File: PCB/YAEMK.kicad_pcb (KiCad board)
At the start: 2 copper layers, 162.8 x 130.8 mm, 177 parts, among them J1 DBG, P1 PC, P2 Link, P3 SSD1107, Q1 SSP6206, SW1 ALPS EC11, U1 USBLC6-2SC6, U2 USBLC6-2SC6, U3 STM32F103CBTx

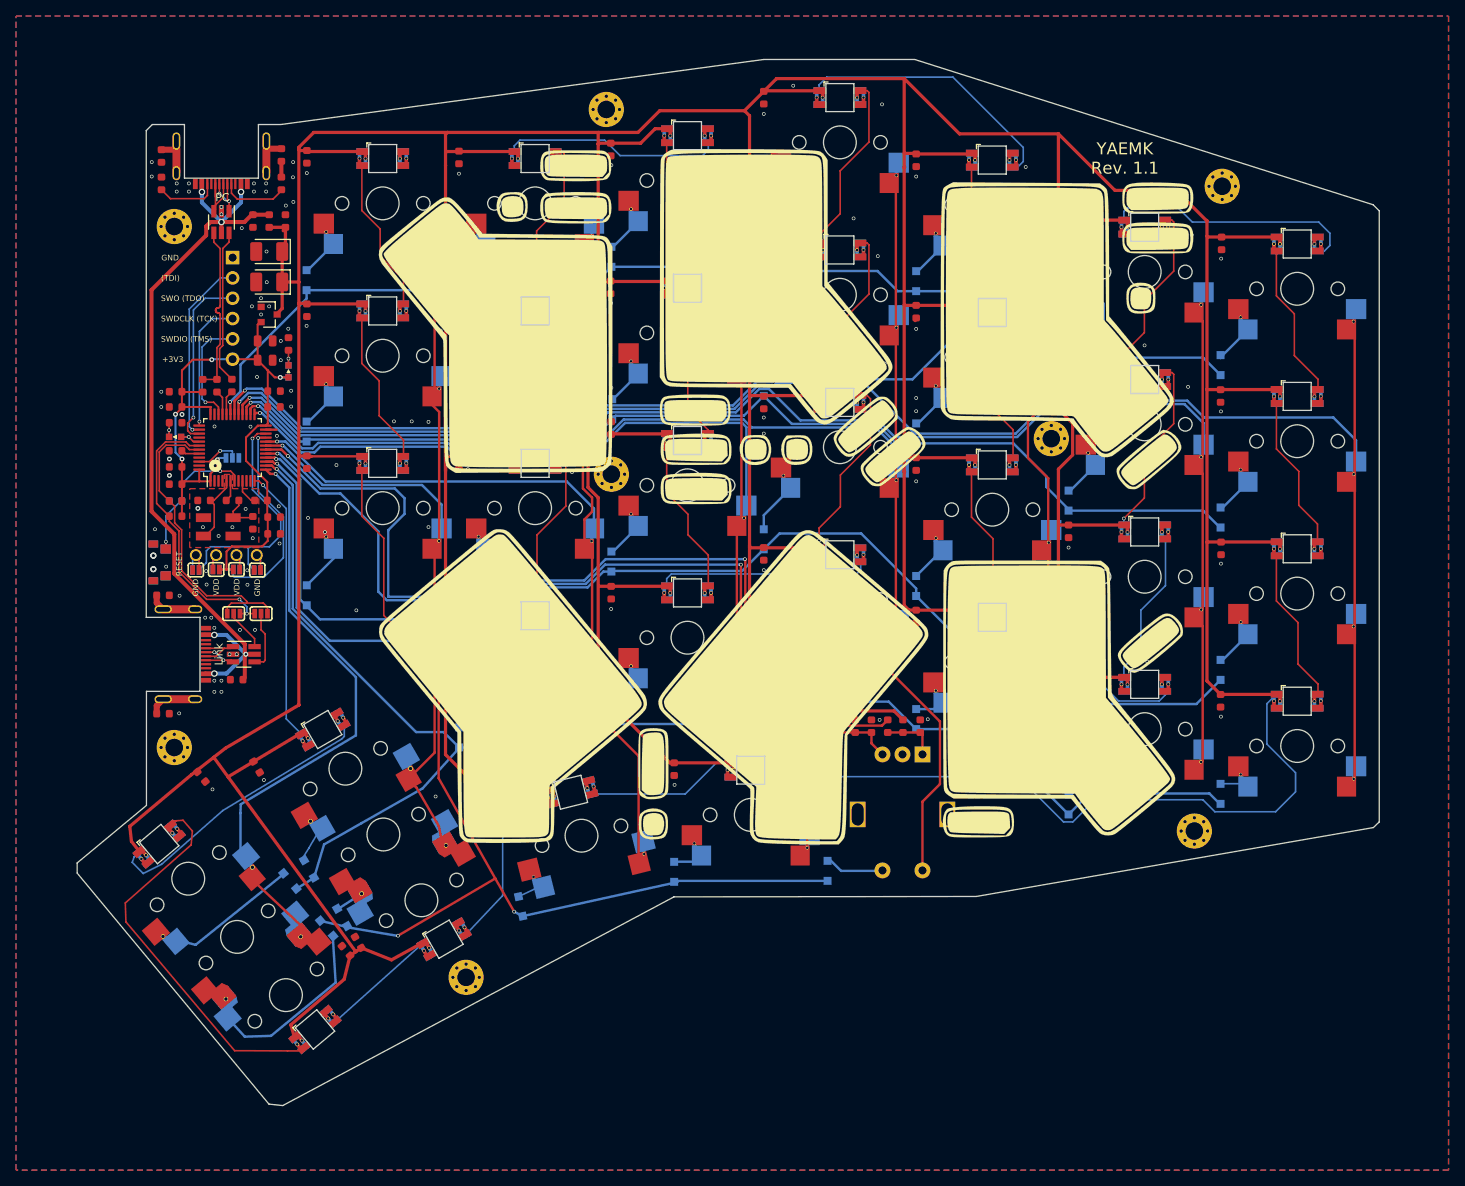
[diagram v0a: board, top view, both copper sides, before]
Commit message: Add WIP yaemk 1.2 files
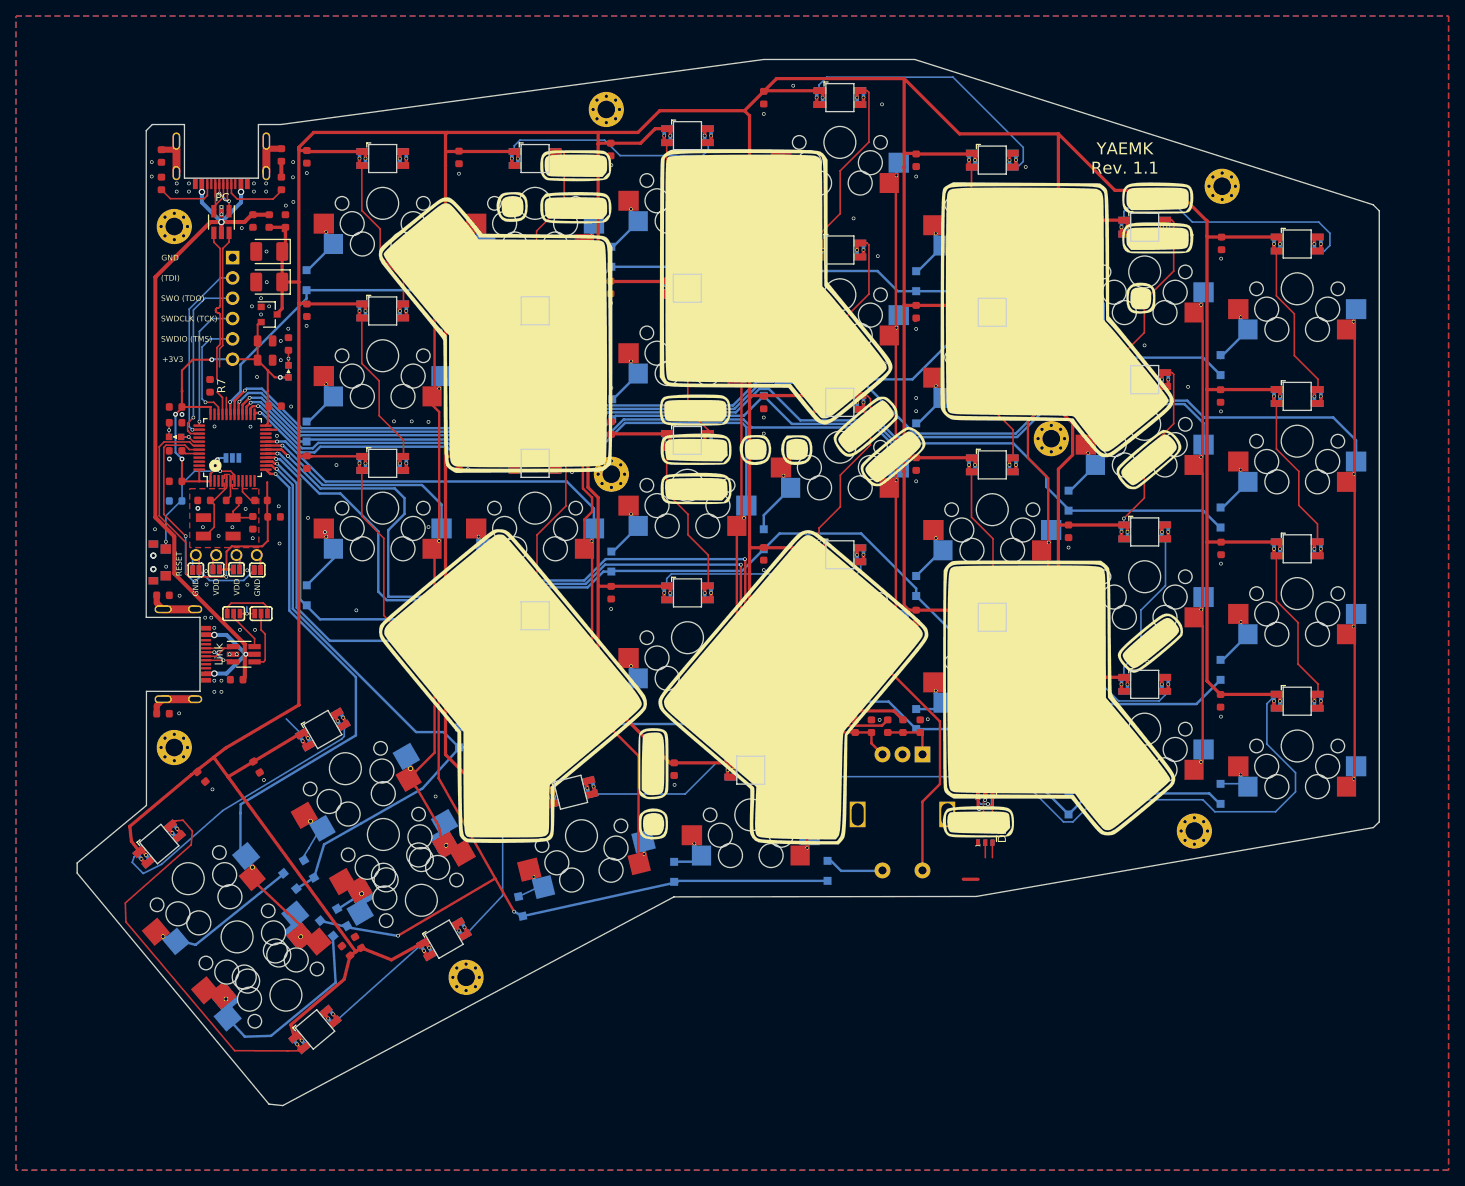
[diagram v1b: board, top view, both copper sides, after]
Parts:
- removed C3, C38, C50, C52: 100n, prettylib:SMD-0603
- removed R14: 1k5, prettylib:SMD-0603
- removed R15, R16: 2k2, prettylib:SMD-0603
- removed R8: 33, prettylib:SMD-0603
- added D28: APA102-2020, prettylib:LED-APA102-2020, F.Cu at (182.0, 124.0)
- added D8: APA102-2020, prettylib:LED-APA102-2020, F.Cu at (182.0, 118.1)
- HSE1: value 12MHz -> 8MHz
- R7: value 33 -> 1k5
- S10, S11, S12, S13, S14, S15, S16, S17, S18, S19, S2, S20, S21, S22, S24, S25, S26, S27, S28, S29, S3, S30, S31, S32, S33, S34, S35, S4, S9: footprint prettylib:MX_KAILH_SOCKET_WS2812_1U -> prettylib:MX_KAILH_SOCKET_SK9822_1U
- moved C45 15.8 mm to (93.2, 70.7), turned to 0 degrees
- moved R7 2.73 mm to (85.1, 68.2), turned to 270 degrees
- moved C47 2.12 mm to (93.1, 84.6)
- moved C43 1.80 mm to (80.8, 80.1)
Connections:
- JP1 pad 1: USART1_RX -> USART3_RX
- JP1 pad 3: USART1_TX -> USART3_TX
- JP11 pad 2: HANDNESS -> (no net)
- JP2 pad 1: USART1_RX -> USART3_RX
- JP2 pad 3: USART1_TX -> USART3_TX
- JP3 pad 1: I2C2_SDA -> I2C1_SDA
- JP4 pad 1: I2C2_SCL -> I2C1_SCL
- JP7 pad 1: I2C2_SDA -> I2C1_SDA
- JP8 pad 1: I2C2_SCL -> I2C1_SCL
- R7 pad 1: Net-(R7-Pad1) -> USB_D+
- R7 pad 2: USB_D- -> VDD
- U3 pad 12: TIM2_CH3 -> (no net)
- U3 pad 21: I2C2_SCL -> USART3_TX
- U3 pad 22: I2C2_SDA -> USART3_RX
- U3 pad 26: Col5 -> (no net)
- U3 pad 28: Col7 -> (no net)
- U3 pad 32: Net-(R7-Pad1) -> USB_D-
- U3 pad 33: Net-(R8-Pad2) -> USB_D+
- U3 pad 42: USART1_TX -> I2C1_SCL
- U3 pad 43: USART1_RX -> I2C1_SDA
- U3 pad 46: HANDNESS -> (no net)
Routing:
- net USART1_RX: track 39.0 -> 0.00 mm
- net USART1_TX: track 35.2 -> 0.00 mm, vias 2 -> 0
- net I2C1_SDA: track 0.00 -> 33.4 mm, vias 0 -> 1
- net I2C2_SDA: track 32.1 -> 0.00 mm, vias 1 -> 0
- net TIM2_CH3: track 34.4 -> 2.65 mm, vias 1 -> 0
- net I2C1_SCL: track 0.00 -> 30.6 mm, vias 0 -> 1
- net I2C2_SCL: track 27.3 -> 0.00 mm, vias 1 -> 0
- net VDD: track 92.4 -> 75.4 mm
- net +5V: track 1018.0 -> 1026.5 mm, vias 0 -> 1
- net USART3_RX: track 0.00 -> 7.53 mm
- net Net-(D28-Pad4): track 0.00 -> 5.90 mm, vias 0 -> 1
- net HANDNESS: track 5.55 -> 0.00 mm, vias 1 -> 0
- net Net-(D28-Pad5): track 0.00 -> 4.43 mm, vias 0 -> 2
- net Net-(R7-Pad1): track 3.10 -> 0.00 mm
- net Net-(R8-Pad2): track 3.07 -> 0.00 mm
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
